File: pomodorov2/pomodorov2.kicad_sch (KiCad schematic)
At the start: 12 parts, among them J1 USB_B_Micro, J2 TC2050-IDC, J3 Conn_01x08, U1 MDBT50Q-1MV2, Y1 32.768kHz

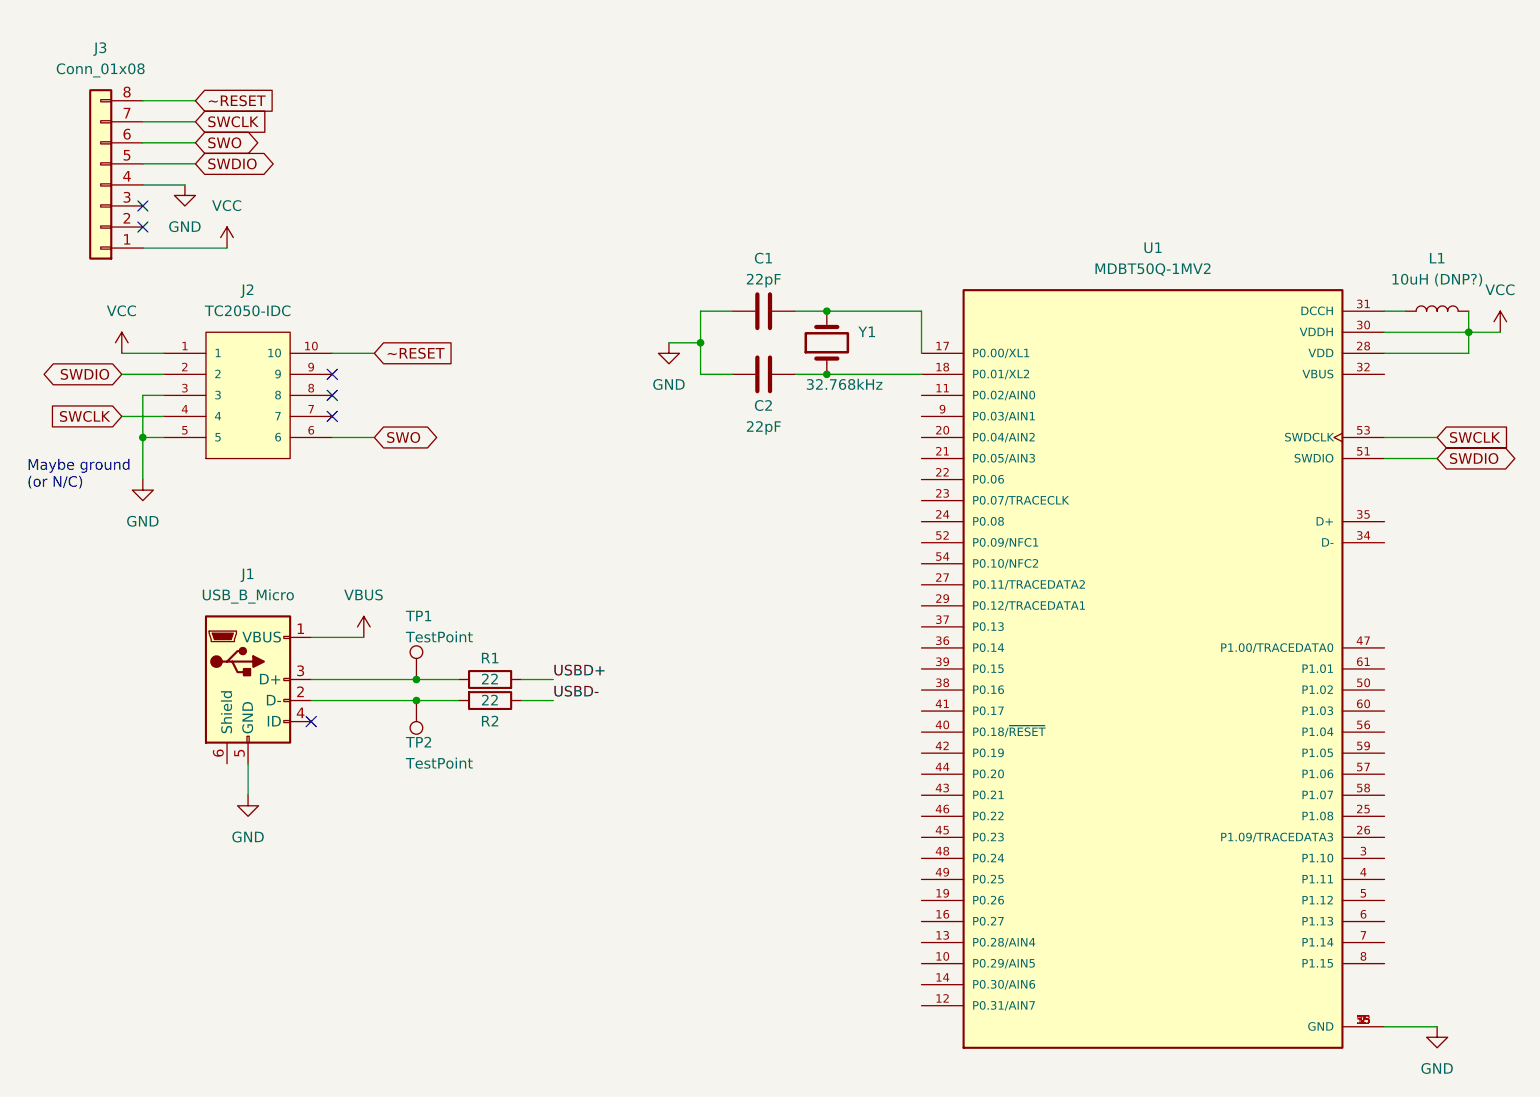
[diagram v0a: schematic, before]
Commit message: A little routing and schematic cleanup 🧹
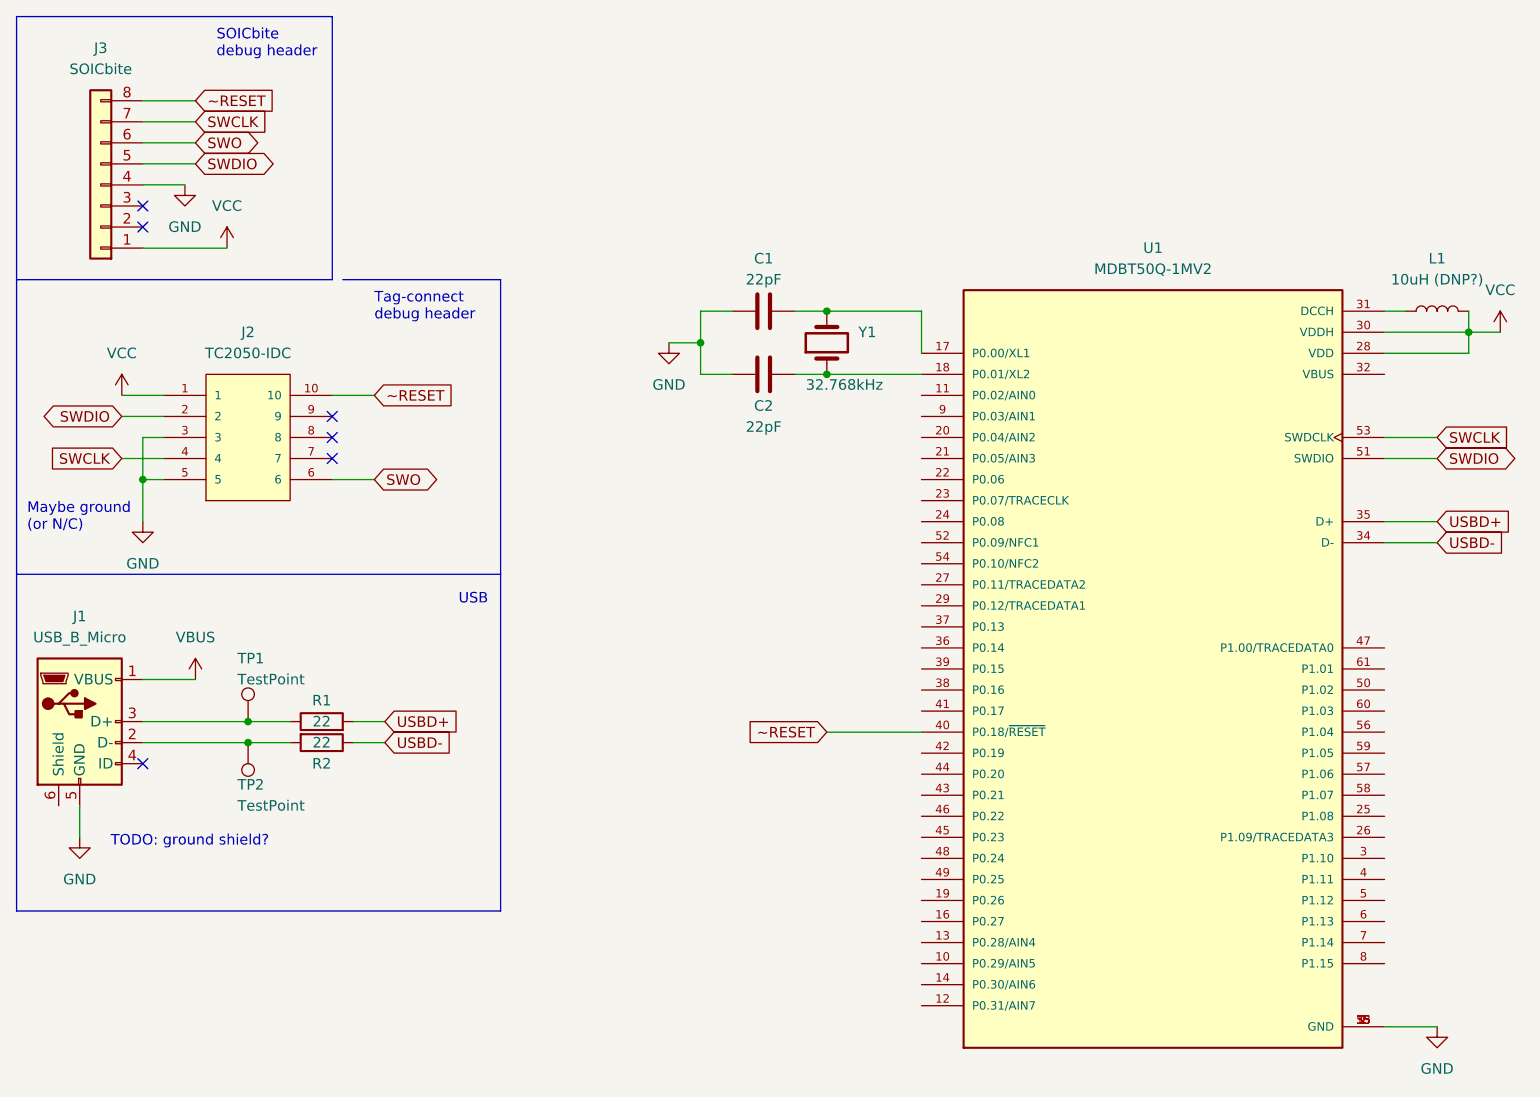
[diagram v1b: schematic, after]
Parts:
- J3: value Conn_01x08 -> SOICbite
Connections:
- net USBD+: now also U1.35 (D+)
- net USBD-: now also U1.34 (D-)
- net ~RESET: now also U1.40 (P0.18/~{RESET})
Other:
- note added: "SOICbite debug header"
- note added: "TODO: ground shield?"
- note added: "Tag-connect debug header"
- note added: "USB"
- moved on the sheet: J1, J2, R1, R2, TP1, TP2
